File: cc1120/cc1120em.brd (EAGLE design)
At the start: 39.4 x 35.6 mm, 40 parts, among them U1 CC1120_RHM_32, X1 FA-128

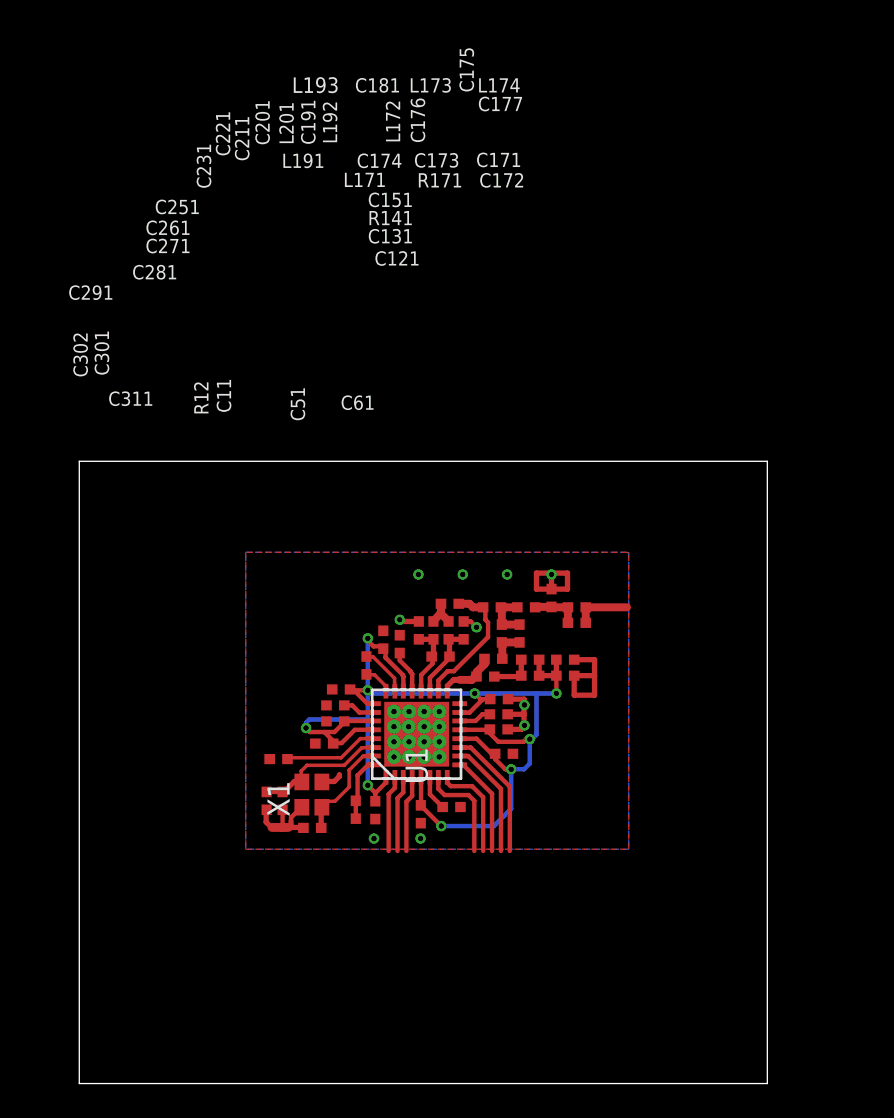
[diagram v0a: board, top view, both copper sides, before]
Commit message: Work on CC2538 Z1 board
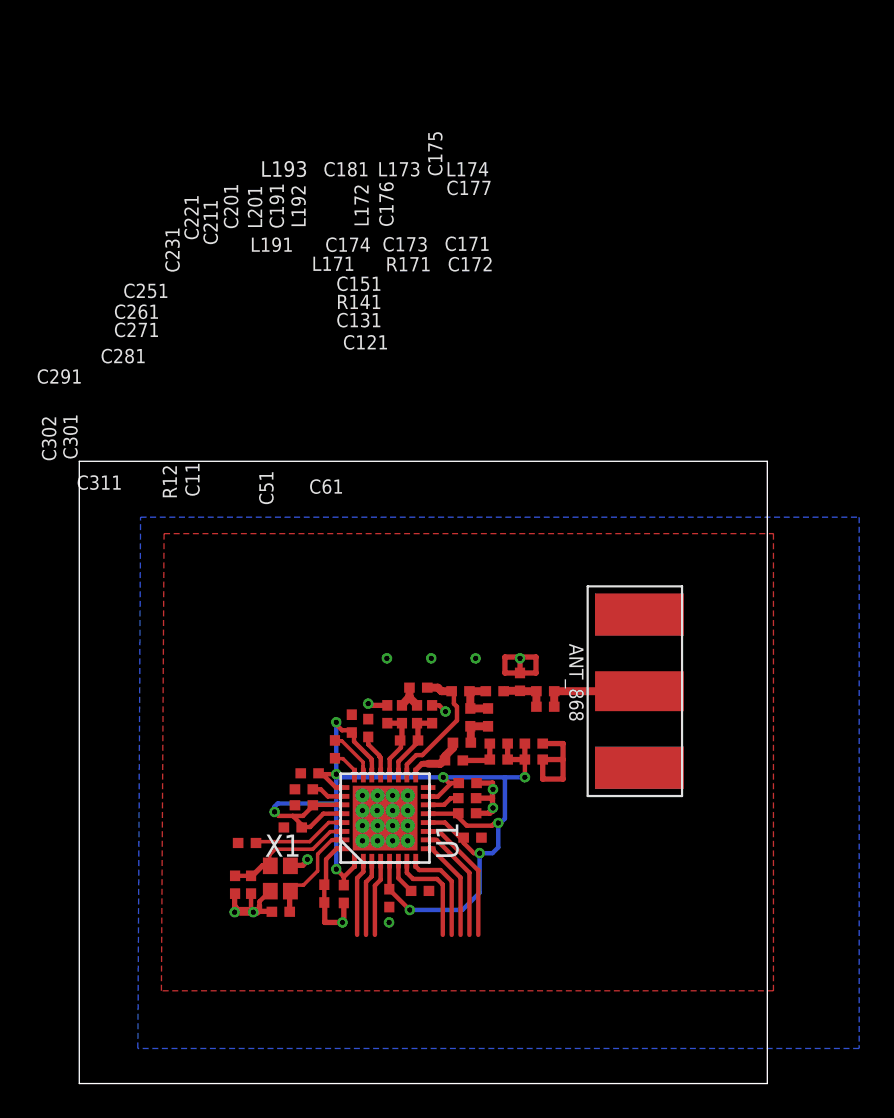
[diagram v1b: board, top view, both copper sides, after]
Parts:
- added ANT_868: SMA, CC11x:JOHNSON_142-0701-806
- moved C151 5.13 mm to (22.3, 17.2)
- moved C171 5.13 mm to (26.0, 19.5)
- moved C173 5.13 mm to (24.0, 19.5)
- moved C177 5.13 mm to (26.7, 21.6)
- moved C231 5.13 mm to (14.6, 19.2)
- moved C11 5.13 mm to (15.1, 10.8)
- moved C131 5.13 mm to (22.2, 15.5)
- moved C271 5.13 mm to (12.8, 15.9)
- moved R12 5.13 mm to (14.0, 10.9)
- moved C221 5.13 mm to (15.6, 20.6)
- moved C291 5.13 mm to (9.58, 13.8)
- moved C121 5.13 mm to (22.5, 14.1)
- moved C172 5.13 mm to (26.0, 18.5)
- moved C174 5.13 mm to (21.9, 19.5)
- moved C175 5.13 mm to (25.2, 23.0)
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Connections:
- new net 3: ANT_868.3
- new net 4: ANT_868.4
- net GND: now also ANT_868.1, ANT_868.2, U1.V, U1.V_10, U1.V_11, U1.V_12, U1.V_13, U1.V_14, U1.V_15, U1.V_16, U1.V_2, U1.V_3, U1.V_4, U1.V_5, U1.V_6, U1.V_7, U1.V_8, U1.V_9
- net N$18: now also ANT_868.RF
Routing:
- net GND: track 30.5 -> 34.0 mm, vias 10 -> 13
- net N$18: track 3.25 -> 5.76 mm
